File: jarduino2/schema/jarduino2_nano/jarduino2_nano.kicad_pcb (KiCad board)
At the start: 2 copper layers, 118 x 95 mm, 42 parts, among them J1 Power, J2 Interface, J3 Pompe 1, J4 Pompe 2, J5 Ext Ser, Q1 Q_NPN_BCE, Q2 Q_NPN_BCE, U1 RFB-0505S, U2 RtcArduino, U3 DHT22

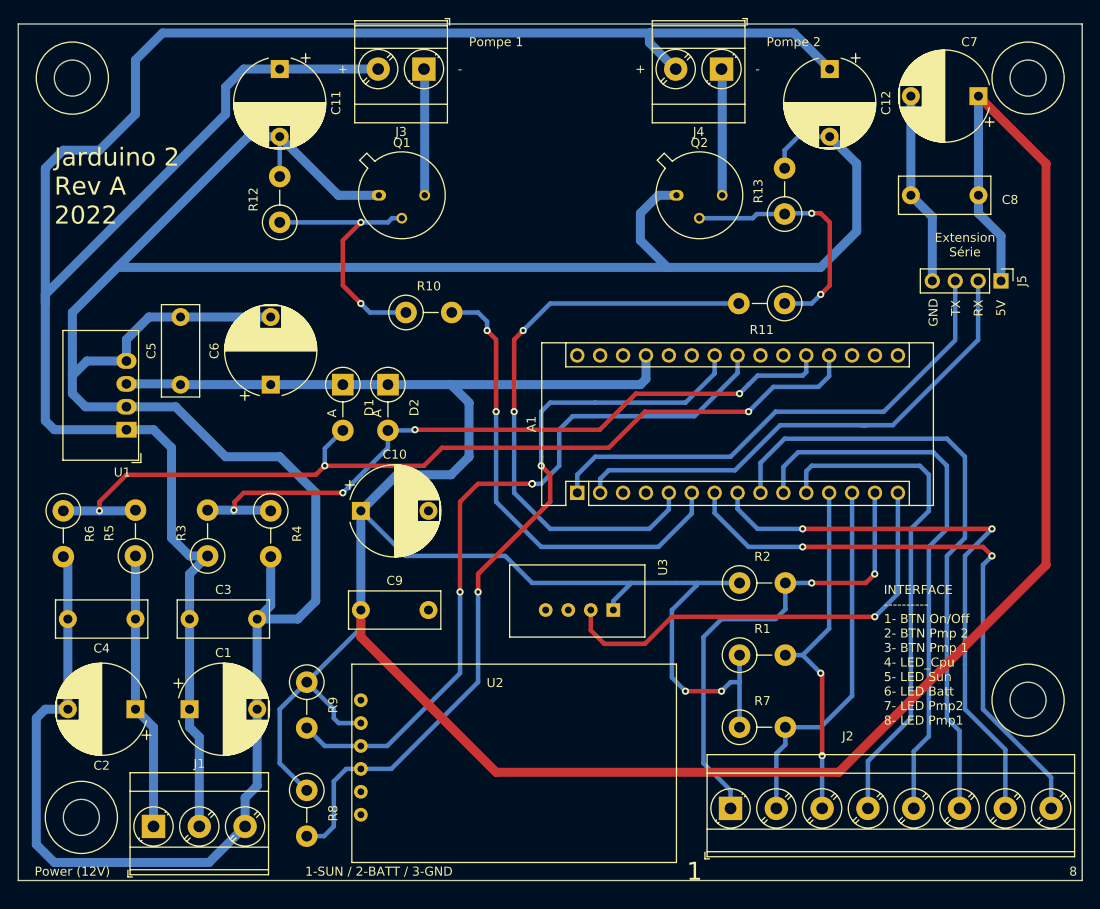
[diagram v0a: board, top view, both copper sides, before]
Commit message: Amélioration 3d / libs
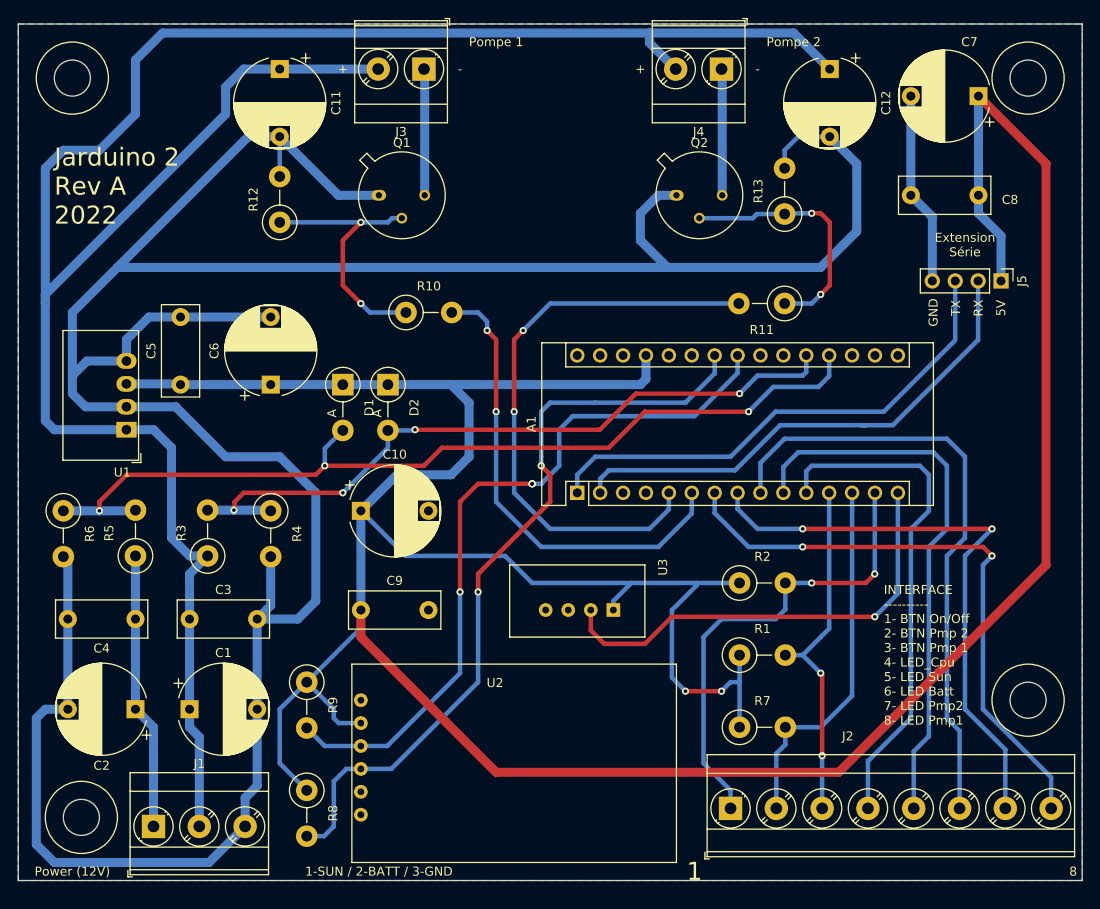
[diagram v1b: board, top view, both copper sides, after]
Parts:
- A1: footprint Module:Arduino_Nano -> bpc:BPC_Arduino_Nano
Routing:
- added copper zone on B.Cu, net GND
